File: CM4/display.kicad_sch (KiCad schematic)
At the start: 1 part, among them J6 ZF5S-20-01-T-WT

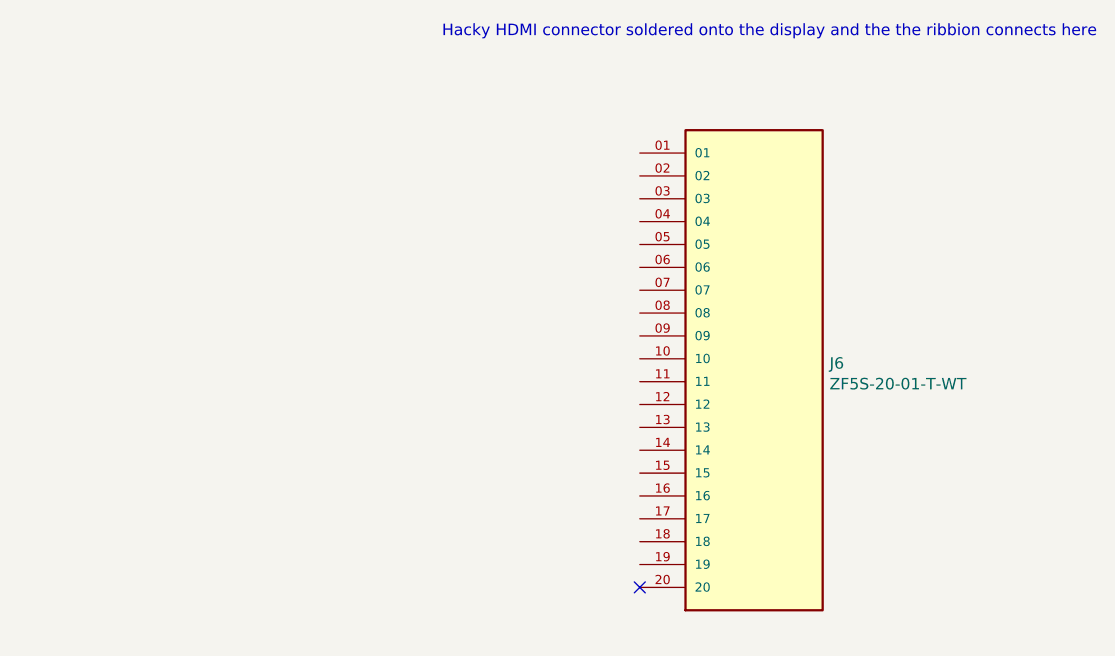
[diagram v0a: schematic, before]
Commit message: PrepedHDMIConnections
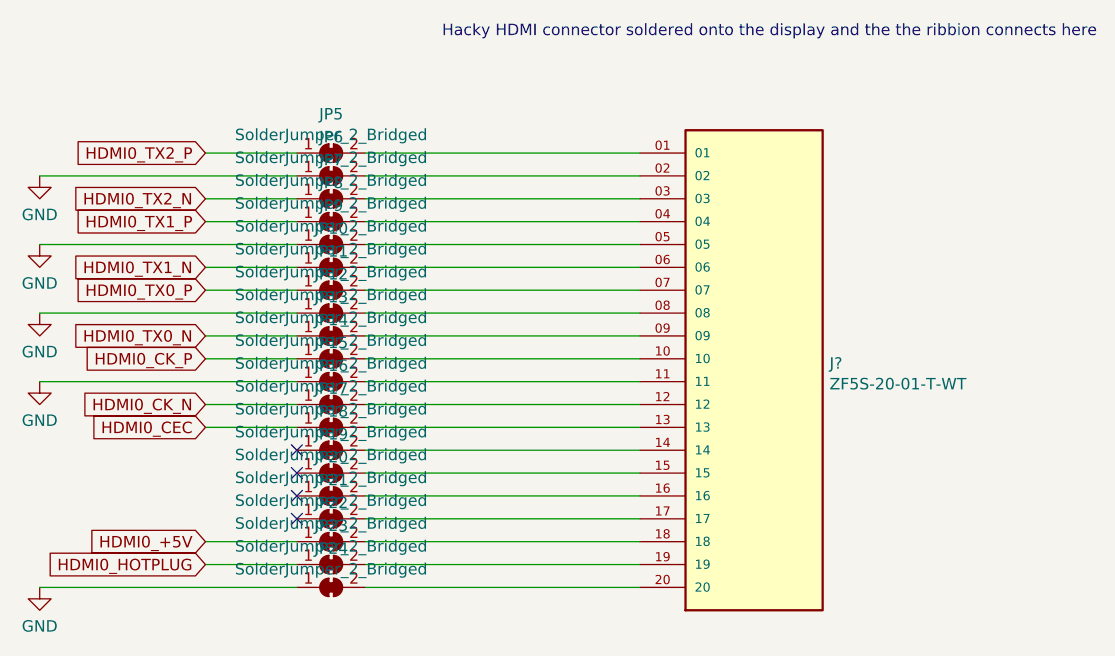
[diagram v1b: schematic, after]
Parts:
- removed J6: ZF5S-20-01-T-WT, SAMTEC_ZF5S-20-01-T-WT, symbol ZF5S-20-01-T-WT:ZF5S-20-01-T-WT
- added J?: ZF5S-20-01-T-WT, SAMTEC_ZF5S-20-01-T-WT, symbol ZF5S-20-01-T-WT:ZF5S-20-01-T-WT
- added JP10, JP11, JP12, JP13, JP14, JP15, JP16, JP17, JP18, JP19, JP20, JP21, JP22, JP23, JP5, JP6, JP7, JP8, JP9: SolderJumper_2_Bridged, Jumper:SolderJumper-2_P1.3mm_Bridged_Pad1.0x1.5mm, symbol Jumper:SolderJumper_2_Bridged
- added JP24: SolderJumper_2_Bridged, symbol Jumper:SolderJumper_2_Bridged
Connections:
- new net: J?.04, JP8.2 (B)
- new net: J?.01, JP5.2 (B)
- new net: J?.02, JP6.2 (B)
- new net: J?.03, JP7.2 (B)
- new net: J?.05, JP9.2 (B)
- new net: J?.06, JP10.2 (B)
- new net: J?.07, JP11.2 (B)
- new net: J?.08, JP12.2 (B)
- new net: J?.09, JP13.2 (B)
- new net: J?.10, JP14.2 (B)
- new net: J?.11, JP15.2 (B)
- new net: J?.12, JP16.2 (B)
- new net: J?.13, JP17.2 (B)
- new net: J?.14, JP18.2 (B)
- new net: J?.15, JP19.2 (B)
- new net: J?.16, JP20.2 (B)
- new net: J?.17, JP21.2 (B)
- new net: J?.18, JP22.2 (B)
- new net: J?.19, JP23.2 (B)
- new net: J?.20, JP24.2 (B)
- new net GND: JP12.1 (A), JP15.1 (A), JP24.1 (A), JP6.1 (A), JP9.1 (A)
- new net HDMI0_+5V: JP22.1 (A)
- new net HDMI0_CEC: JP17.1 (A)
- new net HDMI0_CK_N: JP16.1 (A)
- new net HDMI0_CK_P: JP14.1 (A)
- new net HDMI0_HOTPLUG: JP23.1 (A)
- new net HDMI0_TX0_N: JP13.1 (A)
- new net HDMI0_TX0_P: JP11.1 (A)
- new net HDMI0_TX1_N: JP10.1 (A)
- new net HDMI0_TX1_P: JP8.1 (A)
- new net HDMI0_TX2_N: JP7.1 (A)
- new net HDMI0_TX2_P: JP5.1 (A)
- no-connect marks 1 -> 4
